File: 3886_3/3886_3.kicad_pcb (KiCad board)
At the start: 2 copper layers, 95 x 78 mm, 59 parts, among them J101 2, J102 2, J103 3, Q101 BT139-600E, Q102 BC817, Q103 BC807, U101 LM3886TF

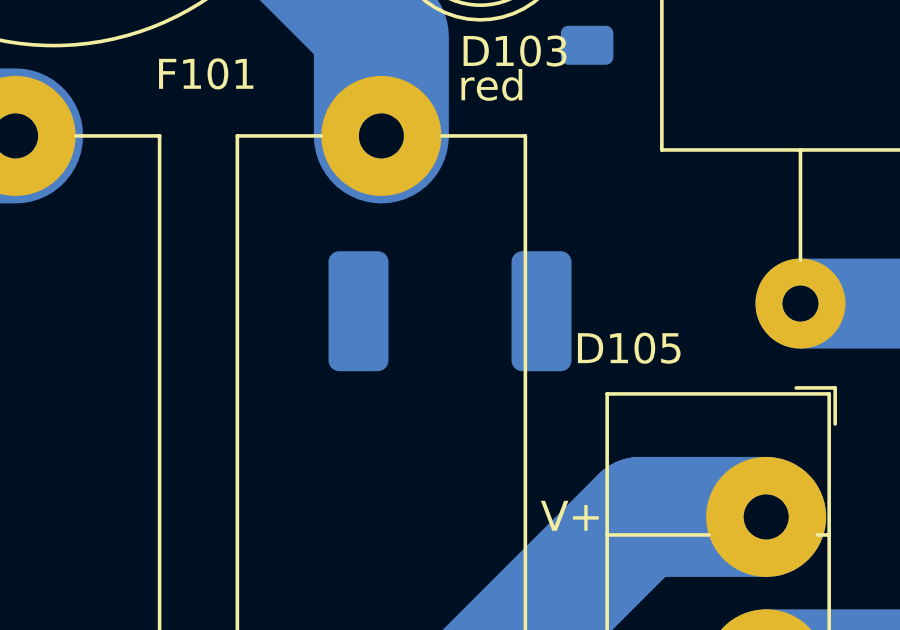
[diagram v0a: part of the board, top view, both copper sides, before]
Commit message: Add files via upload
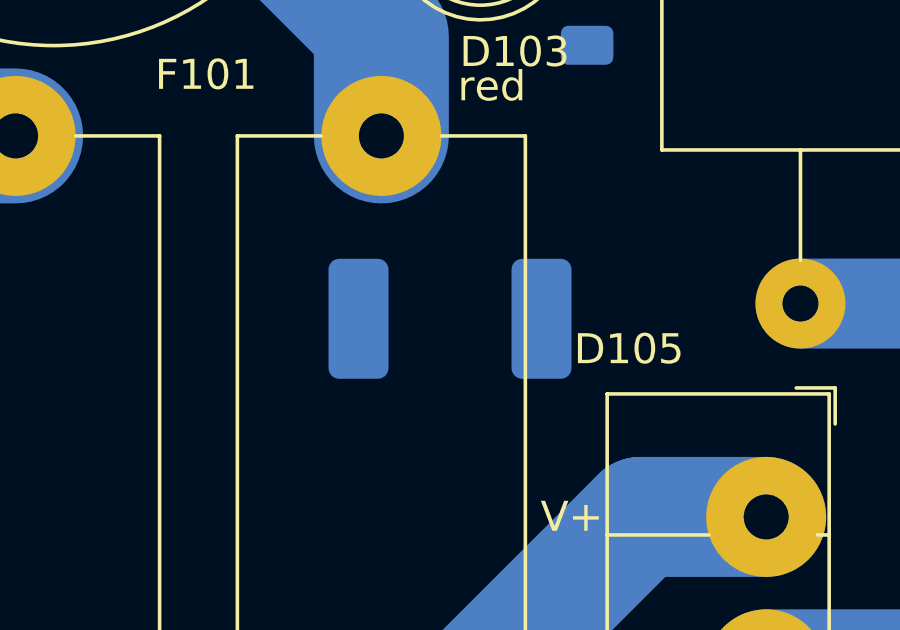
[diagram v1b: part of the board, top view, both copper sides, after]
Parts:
- moved R121 0.25 mm to (51.3, 91.7)
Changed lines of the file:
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@@
 	(footprint "Resistor_SMD:R_2512_6332Metric_Pad1.40x3.35mm_HandSolder"
 		(layer "B.Cu")
-		(at 51.31 91.44 180)
+		(at 51.31 91.694 180)
 		(descr "Resistor SMD 2512 (6332 Metric), square (rectangular) end terminal, IPC-7351 nominal with elongated pad for handsoldering. (Body size source: IPC-SM-782 page 72, https://www.pcb-3d.com/wordpress/wp-content/uploads/ipc-sm-782a_amendment_1_and_2.pdf), generated with kicad-footprint-generator")
 		(tags "resistor handsolder")
